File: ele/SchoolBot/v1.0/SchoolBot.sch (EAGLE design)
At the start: 63 parts, among them X1 M8, X2 M8, X4 POWER_IN

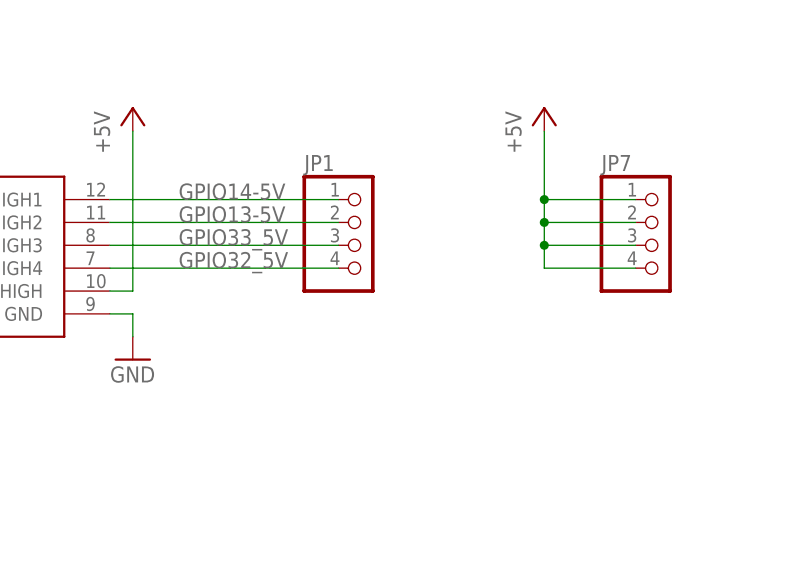
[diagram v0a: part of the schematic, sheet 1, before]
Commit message: new board
-komplenti prekreslini desky
-doplneni rady pinhedu gnd pro 5v piniste
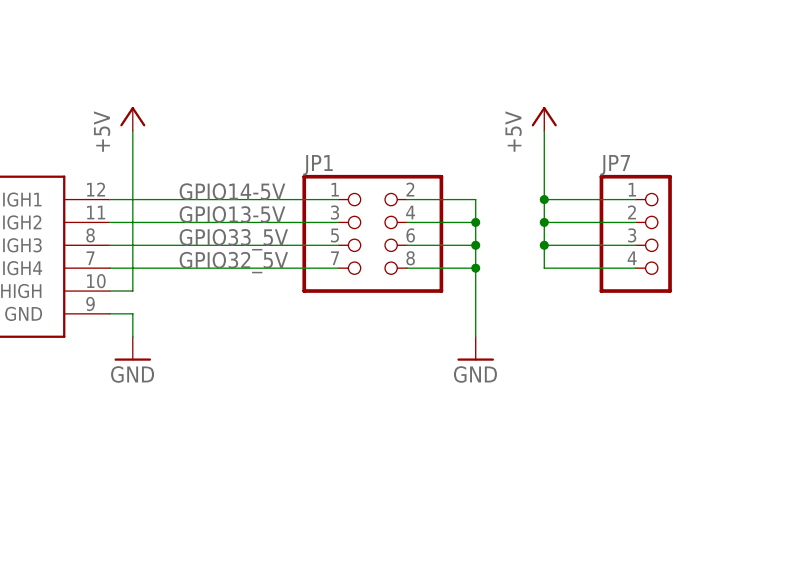
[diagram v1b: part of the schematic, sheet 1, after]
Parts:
- JP1: device pinhead:PINHD-1X4 -> pinhead:PINHD-2X4
- JP7: device pinhead:PINHD-1X4/90 -> pinhead:PINHD-1X4
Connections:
- net GND: now also JP1.2, JP1.4, JP1.6, JP1.8
- net GPIO13-5V: now also JP1.3; no longer JP1.2
- net GPIO32_5V: now also JP1.7; no longer JP1.4
- net GPIO33_5V: now also JP1.5; no longer JP1.3
